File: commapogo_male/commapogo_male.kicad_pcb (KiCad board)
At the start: 4 copper layers, 40.6 x 22.2 mm, 6 parts, among them J1 Conn_02x07_Row_Letter_Last, J2 Conn_02x12_Row_Letter_Last

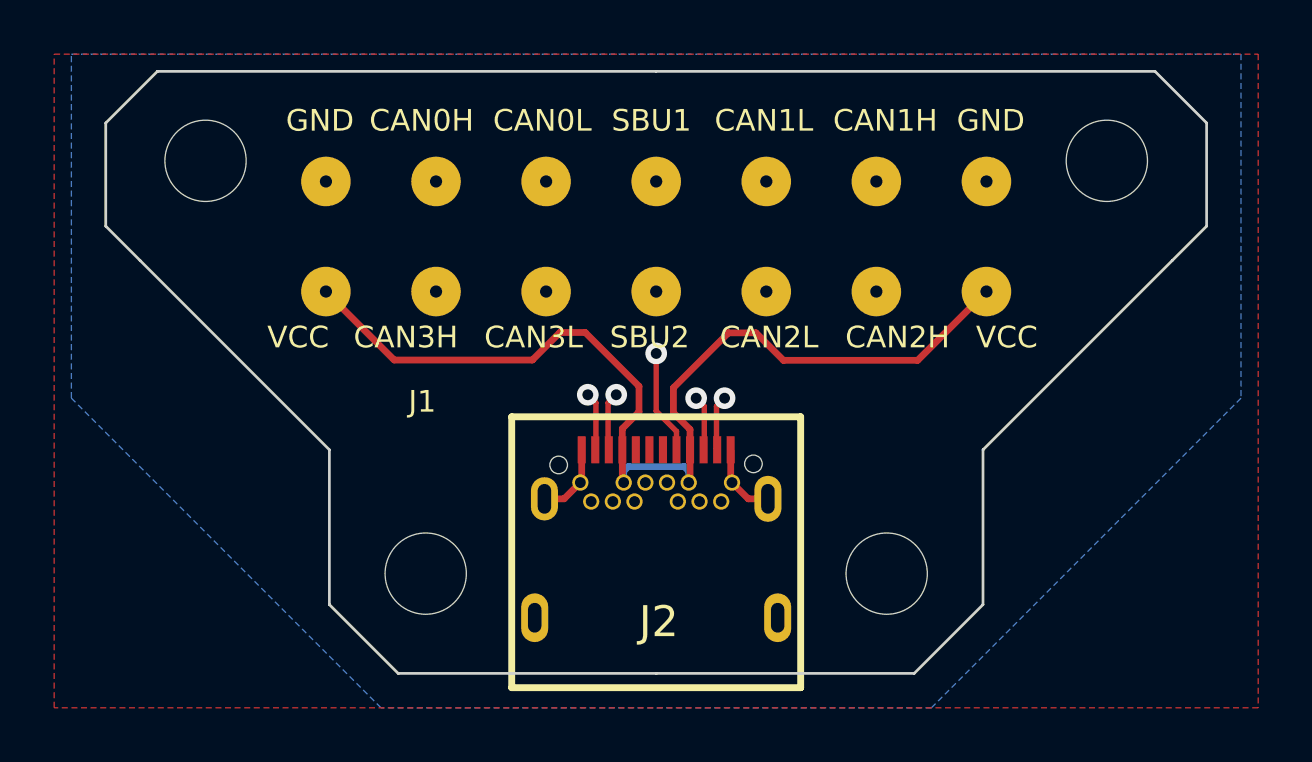
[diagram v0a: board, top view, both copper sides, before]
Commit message: revamp pcb design
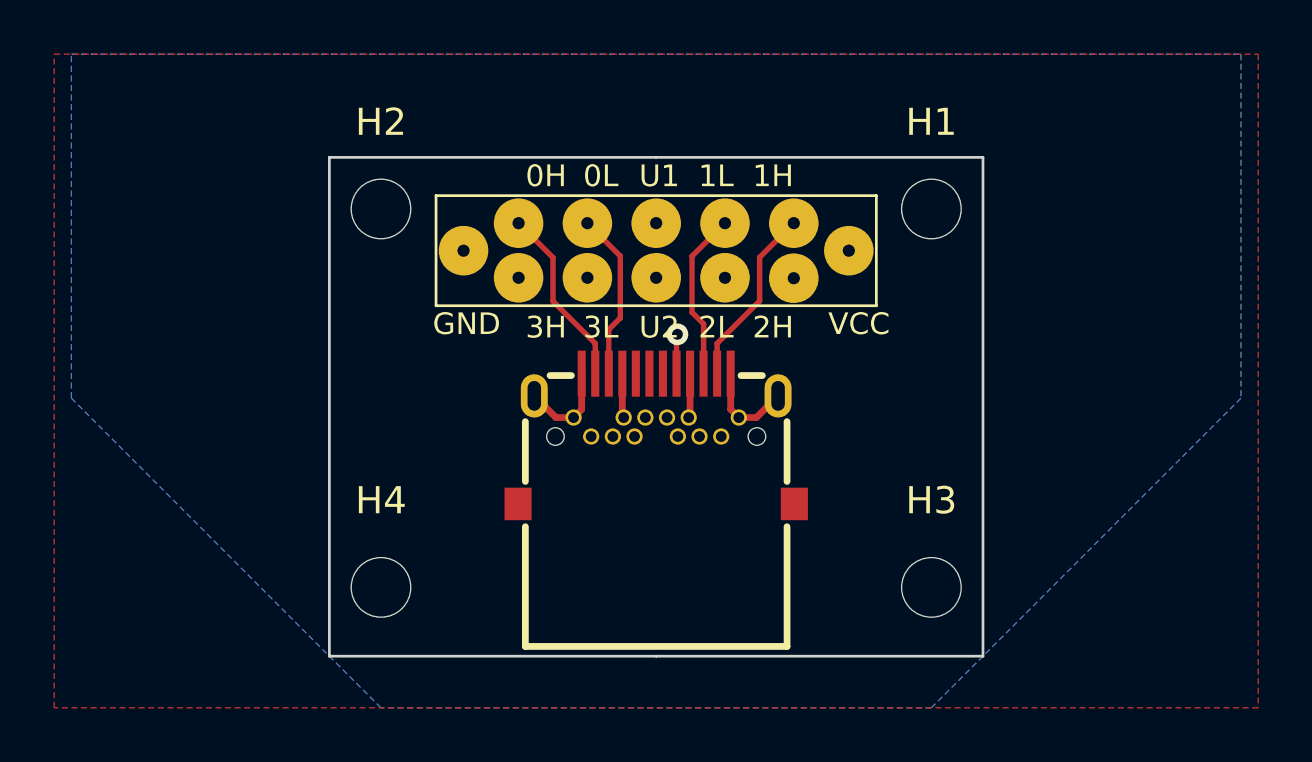
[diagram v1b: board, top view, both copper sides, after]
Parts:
- H1, H2, H3, H4: footprint MountingHole:MountingHole_3mm -> MountingHole:MountingHole_2.2mm_M2
- J2: footprint CommaPogo_Library:USB-C-SMD_HC005-1A1H1A103-0HR -> CommaPogo_Library:GT-USB-7001C
- moved H1 26.9 mm to (150.5, 78.7)
- moved H2 26.9 mm to (130.2, 78.7)
- moved H3 18.7 mm to (150.5, 92.7)
- moved H4 18.7 mm to (130.2, 92.7)
- moved J2 3.50 mm to (140.3, 87.2)
- moved J1 1.54 mm to (140.3, 85.4)
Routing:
- net +12V: track 38.7 -> 15.1 mm
- net /CAN1_P: track 13.8 -> 6.73 mm, vias 1 -> 0
- net /CAN0_P: track 13.8 -> 6.73 mm, vias 1 -> 0
- net /SBU1: track 11.2 -> 6.25 mm
- net /CAN0_N: track 11.1 -> 6.24 mm, vias 1 -> 0
- net /CAN1_N: track 11.1 -> 6.24 mm, vias 1 -> 0
- net /CAN2_P: track 10.3 -> 7.10 mm
- net /CAN3_P: track 10.3 -> 7.12 mm
- net /CAN2_N: track 8.77 -> 6.25 mm
- net /CAN3_N: track 8.77 -> 6.89 mm
- net /SBU2: track 15.6 -> 13.9 mm
- net GND: track 5.61 -> 7.05 mm
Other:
- board size 40.6 x 22.2 mm -> 24.1 x 18.4 mm
- board text removed: "GND"
- board text removed: "VCC"
